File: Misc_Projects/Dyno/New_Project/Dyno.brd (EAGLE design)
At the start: 160 x 100 mm, 8 parts

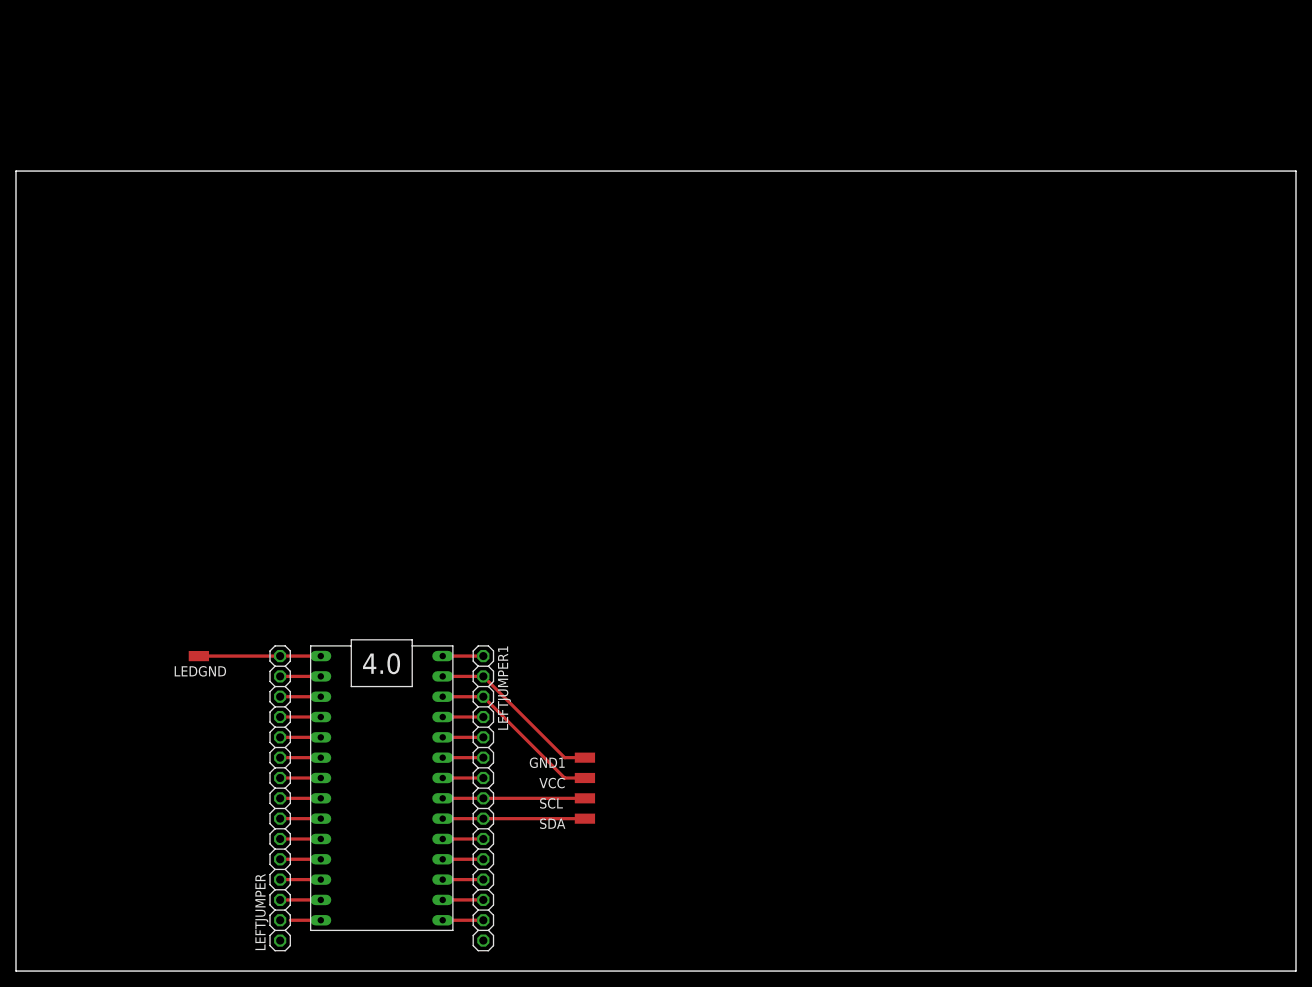
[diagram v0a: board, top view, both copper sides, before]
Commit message: Basic Sch and Board layout
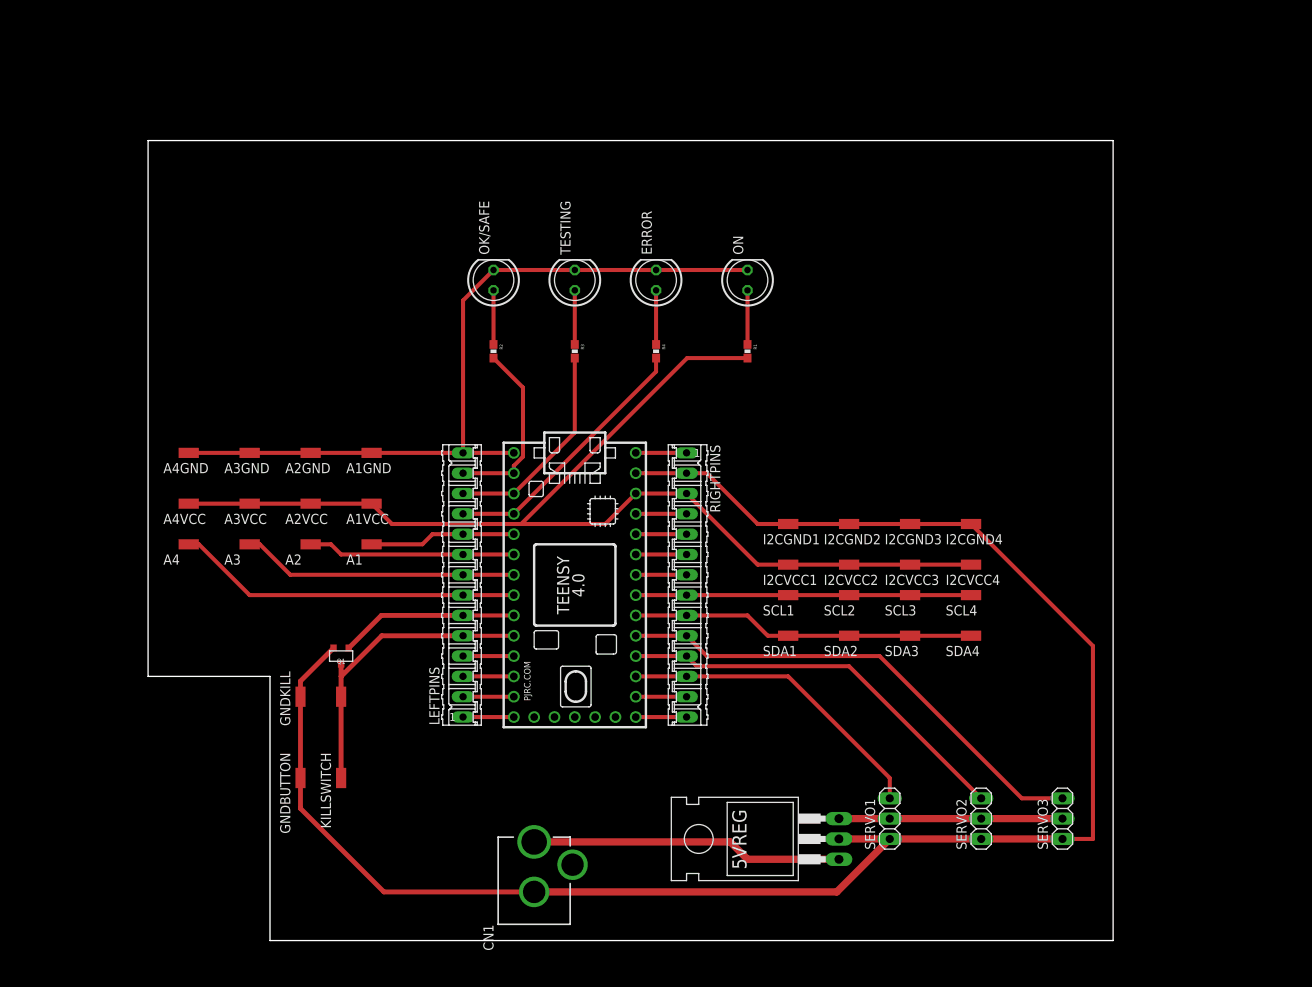
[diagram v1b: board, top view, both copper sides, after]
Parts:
- removed GND1, LEDGND, SCL, SDA, VCC: SOLDER_PAD, HyTechDevices:SOLDER_PAD_XSMALL
- removed LEFTJUMPER, LEFTJUMPER1: (no value), HyTechDevices:1X15
- added 5VREG: (no value), HyTechDevices:TO-220-H
- added A1, A1GND, A1VCC, A2, A2GND, A2VCC, A3, A3GND, A3VCC, A4, A4GND, A4VCC, EMERGENCYSTOPBUTTON, GNDBUTTON, GNDKILL, I2CGND1, I2CGND2, I2CGND3, I2CGND4, I2CVCC1, I2CVCC2, I2CVCC3, I2CVCC4, KILLSWITCH, SCL1, SCL2, SCL3, SCL4, SDA1, SDA2, SDA3, SDA4: SOLDER_PAD, HyTechDevices:SOLDER_PAD_XSMALL
- added CN1: (no value), HyTechDevices:DCJACK_2MM_PTH
- added ERROR: RED, HyTechDevices:LED-5MM
- added LEFTPINS, RIGHTPINS: (no value), con-amp-quick:14P
- added OK/SAFE, ON: GREEN, HyTechDevices:LED-5MM
- added Q1: (no value), HyTechDevices:SOT23
- added R1, R2, R3, R4: (no value), HyTechDevices:0603-RES
- added SERVO1, SERVO2, SERVO3: (no value), HyTechDevices:1X03
- added TESTING: YELLOW, HyTechDevices:LED-5MM
- U$1: value TEENSY_4.0_SIMPLE -> TEENSY_4.0; device HyTechDevices:TEENSY_4.0_SIMPLE -> TEENSY 4.0:TEENSY_4.0
- moved U$1 54.4 mm to (69.8, 48.3), turned to 270 degrees
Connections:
- removed net 3.3V: LEFTJUMPER1.3, U$1.3.3V, VCC.P$1
- removed net N$1: LEFTJUMPER1.1, U$1.VIN
- removed net N$10: LEFTJUMPER.7, U$1.D7(RX2)
- removed net N$17: LEFTJUMPER1.4, U$1.A9
- removed net N$23: LEFTJUMPER1.10, U$1.A3
- removed net N$24: LEFTJUMPER1.11, U$1.A2
- removed net N$25: LEFTJUMPER1.12, U$1.(RX3)A1
- removed net N$26: LEFTJUMPER1.13, U$1.(TX3)A0
- removed net N$3: LEFTJUMPER.14, U$1.D0(RX1)
- removed net N$4: LEFTJUMPER.13, U$1.D1(TX1)
- removed net N$5: LEFTJUMPER.12, U$1.D2
- removed net N$6: LEFTJUMPER.11, U$1.D3
- removed net N$7: LEFTJUMPER.10, U$1.D4
- removed net N$8: LEFTJUMPER.9, U$1.D5
- removed net N$9: LEFTJUMPER.8, U$1.D6
- new net 5V: 5VREG.3, SERVO1.2, SERVO2.2, SERVO3.2
- new net A1PIN3: A1.P$1, LEFTPINS.10, U$1.3/CANTX
- new net A2PIN4: A2.P$1, LEFTPINS.9, U$1.4/CANRX
- new net A3PIN5: A3.P$1, LEFTPINS.8, U$1.5
- new net A4PIN6: A4.P$1, LEFTPINS.7, U$1.6
- new net GNDBREAK: CN1.GNDBREAK
- new net IN: 5VREG.1, CN1.PWR
- new net KILLSWITCH: EMERGENCYSTOPBUTTON.P$1, KILLSWITCH.P$1, LEFTPINS.5, Q1.3, U$1.8
- new net N$21: RIGHTPINS.7, U$1.20/A6
- new net N$28: RIGHTPINS.14, U$1.13/SCK
- new net N$29: ON.A, R1.1
- new net N$30: OK/SAFE.A, R2.1
- new net N$31: R3.1, TESTING.A
- new net N$32: ERROR.A, R4.1
- new net PIN0: LEFTPINS.13, R2.2, U$1.0/RX
- new net PIN1: LEFTPINS.12, R3.2, U$1.1/TX
- new net PIN2: LEFTPINS.11, R4.2, U$1.2
- new net PWM1: RIGHTPINS.12, SERVO1.3, U$1.15/A1
- new net PWM2: RIGHTPINS.11, SERVO2.3, U$1.16/A2
- new net PWM3: RIGHTPINS.10, SERVO3.3, U$1.17/A3
- new net SHUTD: LEFTPINS.6, Q1.1, U$1.7
- new net VCC: A1VCC.P$1, A2VCC.P$1, A3VCC.P$1, A4VCC.P$1, I2CVCC1.P$1, I2CVCC2.P$1, I2CVCC3.P$1, I2CVCC4.P$1, R1.2, RIGHTPINS.3, U$1.3V3_LO
- net GND: now also 5VREG.2, A1GND.P$1, A2GND.P$1, A3GND.P$1, A4GND.P$1, CN1.GND, ERROR.K, GNDBUTTON.P$1, GNDKILL.P$1, I2CGND1.P$1, I2CGND2.P$1, I2CGND3.P$1, I2CGND4.P$1, LEFTPINS.14, OK/SAFE.K, ON.K, Q1.2, RIGHTPINS.2, SERVO1.1, SERVO2.1, SERVO3.1, TESTING.K; no longer GND1.P$1, LEDGND.P$1, LEFTJUMPER.15, LEFTJUMPER1.2
- net N$11: now also LEFTPINS.4, U$1.9/CS; no longer LEFTJUMPER.6, U$1.D8(TX2)
- net N$12: now also LEFTPINS.3, U$1.10/CS; no longer LEFTJUMPER.5, U$1.D9
- net N$13: now also LEFTPINS.2, U$1.11/MOSI; no longer LEFTJUMPER.4, U$1.D10
- net N$14: now also LEFTPINS.1, U$1.12/MISO; no longer LEFTJUMPER.3, U$1.D11
- net N$15: now also RIGHTPINS.1, U$1.VIN; no longer LEFTJUMPER.2, U$1.D12
- net N$18: now also RIGHTPINS.4, U$1.23/A9; no longer LEFTJUMPER1.5, U$1.(CANRX)A8
- net N$19: now also RIGHTPINS.5, U$1.22/A8; no longer LEFTJUMPER1.6, U$1.(CANTX)A7
- net N$20: now also RIGHTPINS.6, U$1.21/A7; no longer LEFTJUMPER1.7, U$1.A6
- net N$27: now also RIGHTPINS.13, U$1.14/A0; no longer LEFTJUMPER1.14, U$1.D13
- net SCL: now also RIGHTPINS.8, SCL1.P$1, SCL2.P$1, SCL3.P$1, SCL4.P$1, U$1.19/A5/SCL; no longer LEFTJUMPER1.8, SCL.P$1, U$1.A5
- net SDA: now also RIGHTPINS.9, SDA1.P$1, SDA2.P$1, SDA3.P$1, SDA4.P$1, U$1.18/A4/SDA; no longer LEFTJUMPER1.9, SDA.P$1, U$1.A4
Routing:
- net GND: track 37.2 -> 320.0 mm
- net VCC: track 0.00 -> 141.0 mm
- net PWM3: track 0.00 -> 61.8 mm
- net PWM2: track 0.00 -> 50.5 mm
- net A4PIN6: track 0.00 -> 43.3 mm
- net PWM1: track 0.00 -> 39.6 mm
- net IN: track 0.00 -> 39.0 mm
- net KILLSWITCH: track 0.00 -> 37.9 mm
- net A3PIN5: track 0.00 -> 34.6 mm
- net PIN2: track 0.00 -> 33.2 mm
- net 5V: track 0.00 -> 27.9 mm
- net PIN1: track 0.00 -> 26.4 mm
- net A2PIN4: track 0.00 -> 25.9 mm
- net SDA: track 17.8 -> 43.0 mm
- net SCL: track 17.8 -> 40.6 mm
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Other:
- board size 160 x 100 mm -> 120.6 x 100 mm

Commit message: Dyno Rev1
Mostly done. Needs small changes.
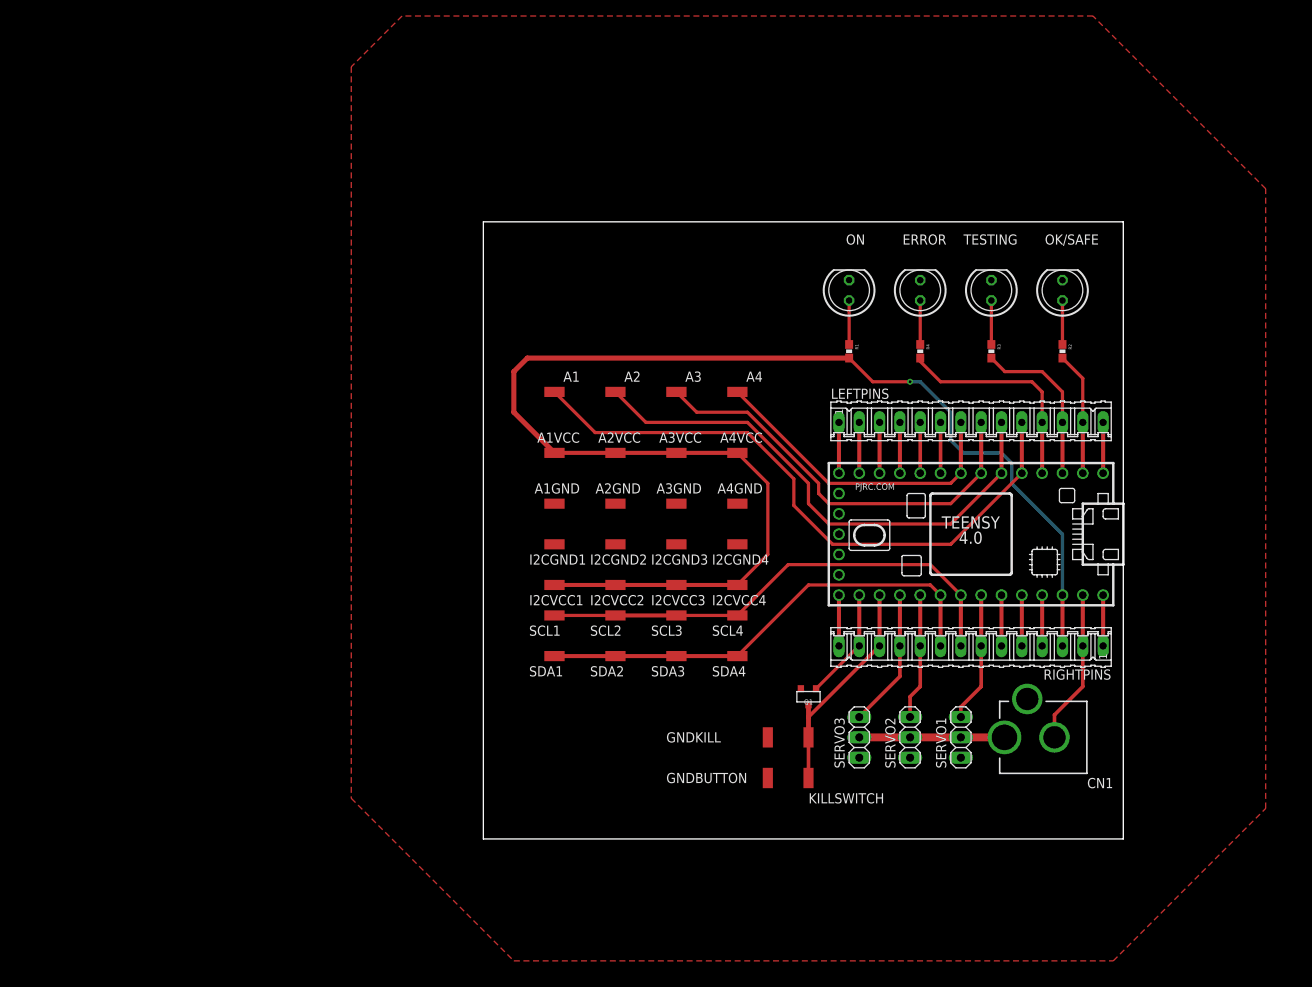
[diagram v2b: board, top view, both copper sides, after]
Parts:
- removed 5VREG: (no value), HyTechDevices:TO-220-H
- moved CN1 77.1 mm to (137.2, 29.2), turned to 90 degrees
- moved A4 71.2 mm to (90.2, 72.4), turned to 180 degrees
- moved OK/SAFE 71.1 mm to (130.8, 85.1)
- moved R2 71.1 mm to (130.8, 77.5)
- moved A4GND 68.9 mm to (90.2, 58.4), turned to 180 degrees
- moved A4VCC 68.9 mm to (90.2, 64.8), turned to 180 degrees
- moved LEFTPINS 66.7 mm to (119.4, 68.6), turned to 0 degrees
- moved EMERGENCYSTOPBUTTON 58.6 mm to (99.1, 29.2)
- moved GNDKILL 58.6 mm to (94.0, 29.2)
- moved Q1 58.6 mm to (99.1, 34.3)
- moved GNDBUTTON 58.4 mm to (94.0, 24.1)
- moved KILLSWITCH 58.4 mm to (99.1, 24.1)
- moved A3 56.6 mm to (82.5, 72.4), turned to 180 degrees
- moved A3GND 53.7 mm to (82.5, 58.4), turned to 180 degrees
- moved A3VCC 53.7 mm to (82.5, 64.8), turned to 180 degrees
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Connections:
- removed net IN: 5VREG.1, CN1.PWR
- removed net N$21: RIGHTPINS.7, U$1.20/A6
- removed net N$27: RIGHTPINS.13, U$1.14/A0
- removed net SHUTD: LEFTPINS.6, Q1.1, U$1.7
- new net N$1: LEFTPINS.6, U$1.7
- new net N$2: LEFTPINS.5, U$1.8
- new net SHUTDSIG: Q1.1, RIGHTPINS.13, U$1.14/A0
- net 5V: now also CN1.PWR; no longer 5VREG.3
- net GND: no longer 5VREG.2
- net KILLSWITCH: now also RIGHTPINS.12, U$1.15/A1; no longer LEFTPINS.5, U$1.8
- net PWM1: now also RIGHTPINS.7, U$1.20/A6; no longer RIGHTPINS.12, U$1.15/A1
- net PWM2: now also RIGHTPINS.10, U$1.17/A3; no longer RIGHTPINS.11, U$1.16/A2
- net PWM3: now also RIGHTPINS.11, U$1.16/A2; no longer RIGHTPINS.10, U$1.17/A3
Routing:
- net GND: track 320.0 -> 25.7 mm
- net A1PIN3: track 18.3 -> 78.3 mm
- net PWM3: track 61.8 -> 17.3 mm
- net A2PIN4: track 25.9 -> 65.6 mm
- net IN: track 39.0 -> 0.00 mm
- net PWM2: track 50.5 -> 15.8 mm
- net VCC: track 141.0 -> 173.5 mm, vias 0 -> 1
- net PWM1: track 39.6 -> 16.3 mm
- net SHUTD: track 22.3 -> 0.00 mm
- net SCL: track 40.6 -> 61.4 mm
- net A3PIN5: track 34.6 -> 52.6 mm
- net SDA: track 43.0 -> 58.8 mm
- net SHUTDSIG: track 0.00 -> 14.0 mm
- net KILLSWITCH: track 37.9 -> 28.1 mm
- net 5V: track 27.9 -> 18.2 mm
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- added copper zone on layer 1, net GND
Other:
- board size 120.6 x 100 mm -> 80 x 77.1 mm
